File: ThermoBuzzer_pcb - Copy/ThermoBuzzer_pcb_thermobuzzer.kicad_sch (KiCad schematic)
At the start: 10 parts, among them SW2 SW_Push

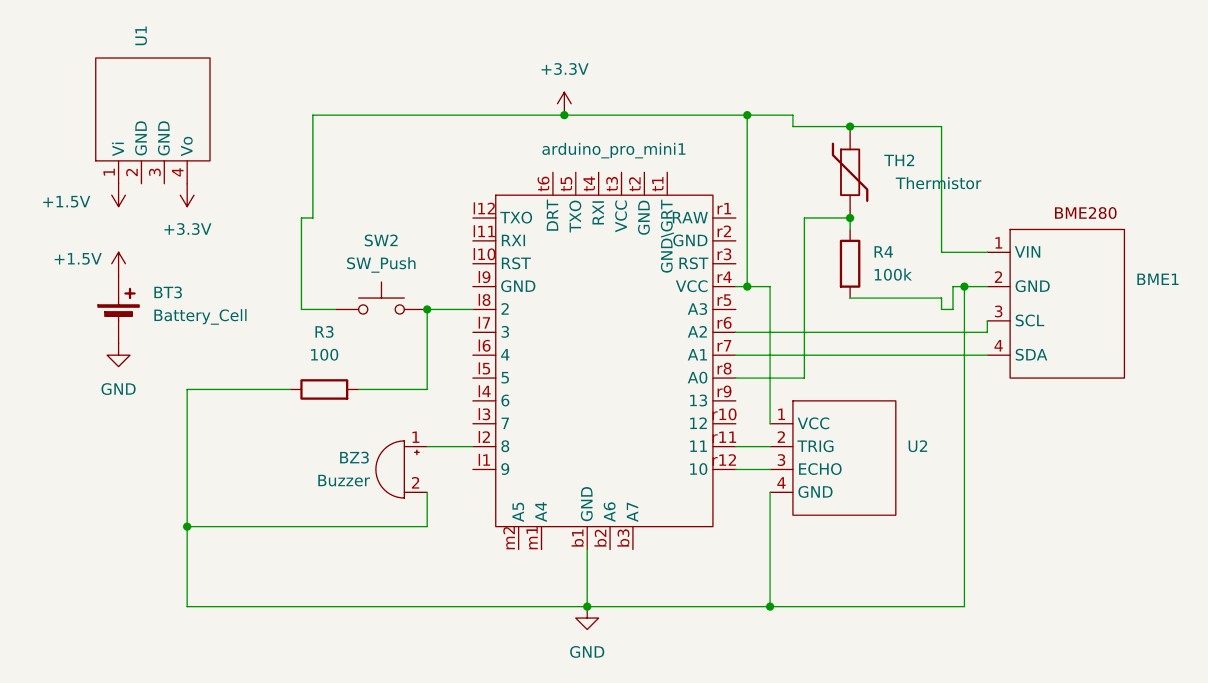
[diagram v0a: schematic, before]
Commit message: 4.21
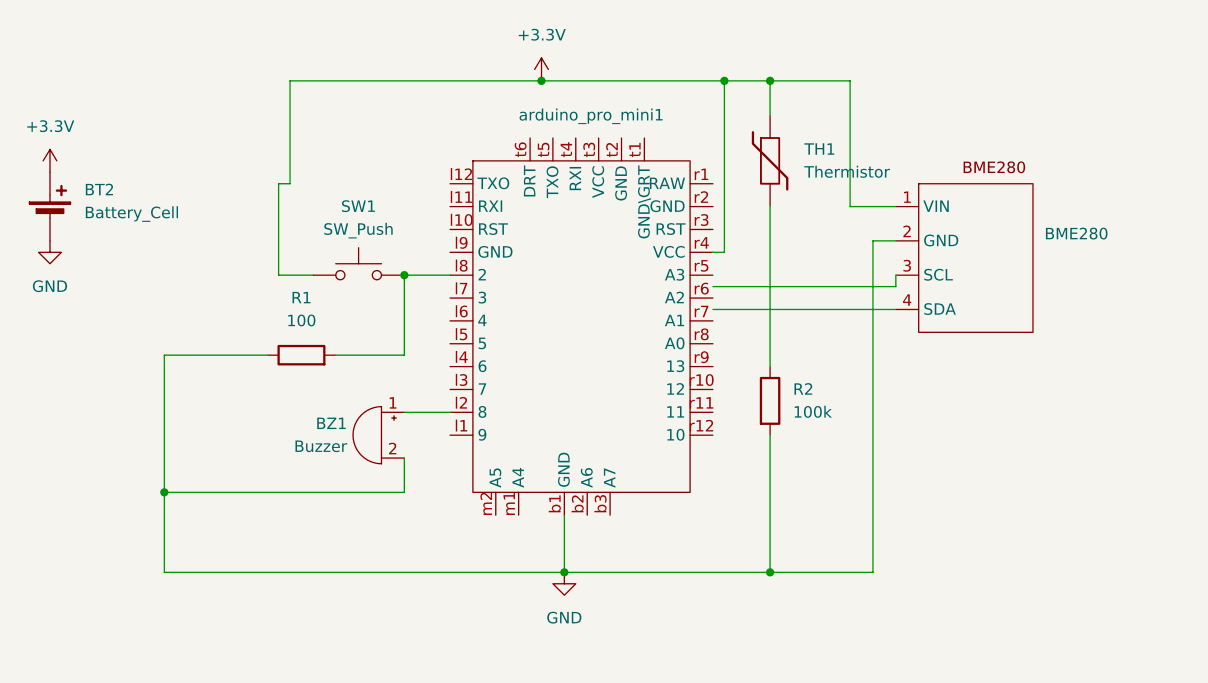
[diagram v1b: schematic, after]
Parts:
- removed BME1: ~, custom_footprints:AHT20+BMP280, symbol thermosensor:BME280_new
- removed BT3: Battery_Cell, Battery:BatteryHolder_Keystone_2460_1xAA, symbol Device:Battery_Cell
- removed BZ3: Buzzer, Buzzer_Beeper:Buzzer_12x9.5RM7.6, symbol Device:Buzzer
- removed R3: 100, Resistor_THT:R_Axial_DIN0207_L6.3mm_D2.5mm_P7.62mm_Horizontal, symbol Device:R
- removed R4: 100k, Resistor_THT:R_Axial_DIN0207_L6.3mm_D2.5mm_P7.62mm_Horizontal, symbol Device:R
- removed SW2: SW_Push, Button_Switch_THT:SW_PUSH_6mm, symbol Switch:SW_Push
- removed TH2: Thermistor, Resistor_THT:R_Axial_DIN0207_L6.3mm_D2.5mm_P7.62mm_Horizontal, symbol Device:Thermistor
- removed U1: ~, custom_footprints:ND0205MA Voltage Regulator, symbol thermosensor:ND0205MA_Voltage_Regulator
- removed U2: ~, custom_footprints:Ultrasonic Sensor HC-SR04, symbol thermosensor:HC-SR04
- added BME280: ~, custom_footprints:AHT20+BMP280, symbol thermosensor:BME280_new
- added BT2: Battery_Cell, Resistor_THT:R_Axial_DIN0204_L3.6mm_D1.6mm_P1.90mm_Vertical, symbol Device:Battery_Cell
- added BZ1: Buzzer, Buzzer_Beeper:Buzzer_12x9.5RM7.6, symbol Device:Buzzer
- added R1: 100, Resistor_THT:R_Axial_DIN0207_L6.3mm_D2.5mm_P7.62mm_Horizontal, symbol Device:R
- added R2: 100k, Resistor_THT:R_Axial_DIN0207_L6.3mm_D2.5mm_P7.62mm_Horizontal, symbol Device:R
- added SW1: SW_Push, Button_Switch_THT:SW_PUSH_6mm, symbol Switch:SW_Push
- added TH1: Thermistor, Resistor_THT:R_Axial_DIN0207_L6.3mm_D2.5mm_P7.62mm_Horizontal, symbol Device:Thermistor
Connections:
- net +3.3V: now also BME280.1 (VIN), BT2.1 (+), SW1.1, TH1.1
- net GND: now also BME280.2 (GND), BT2.2 (-), BZ1.2 (-), R1.1, R2.2
- net at arduino_pro_mini1.l2 (8): now also BZ1.1 (+)
- net at arduino_pro_mini1.l8 (2): now also R1.2, SW1.2
- new net: R2.1, TH1.2
